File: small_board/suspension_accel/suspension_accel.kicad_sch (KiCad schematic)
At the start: 10 parts, among them IC1 TJA1050T_CM,118, IC2 AMS1117-3.3, IC3 ESP32-S3-MINI-1-N8, J1 OSTTE040104

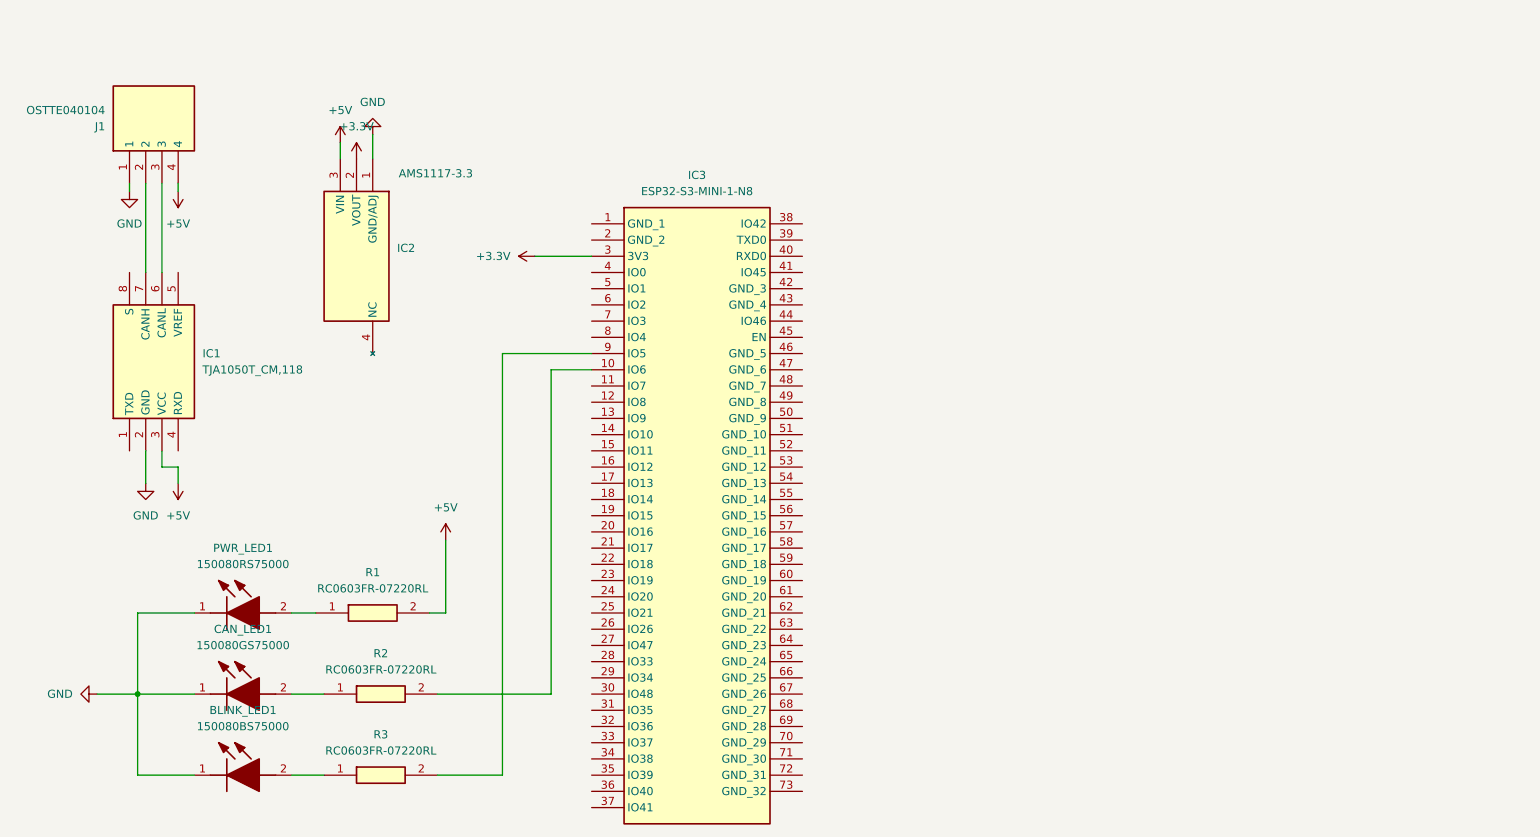
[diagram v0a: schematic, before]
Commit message: small_board work, added buttons
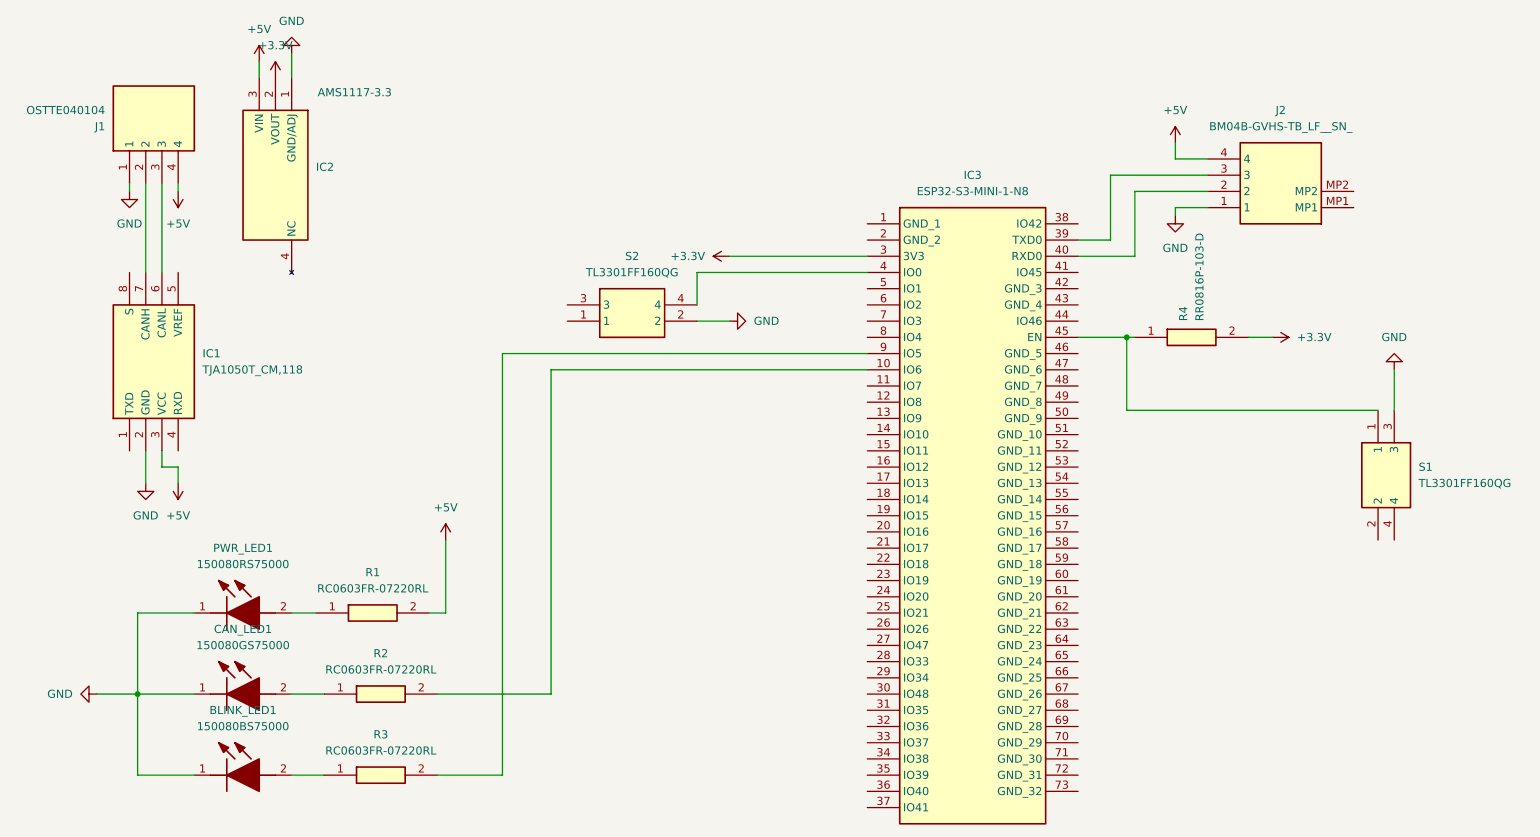
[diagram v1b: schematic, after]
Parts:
- added J2: BM04B-GVHS-TB_LF__SN_, BM04BGVHSTBLFSN, symbol BM04B-GVHS-TB_LF__SN_:BM04B-GVHS-TB_LF__SN_
- added R4: RR0816P-103-D, RESC1608X60N, symbol RR0816P-103-D:RR0816P-103-D
- added S1, S2: TL3301FF160QG, TL3301FF160QG, symbol TL3301FF160QG:TL3301FF160QG
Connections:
- net +3.3V: now also R4.2 (R2)
- net +5V: now also J2.4
- net GND: now also J2.1, S1.3, S2.2
- net at IC3.39 (TXD0): now also J2.3
- net at IC3.4 (IO0): now also S2.4
- net at IC3.40 (RXD0): now also J2.2
- net at IC3.45 (EN): now also R4.1 (R1), S1.1
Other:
- moved on the sheet: IC2, IC3
